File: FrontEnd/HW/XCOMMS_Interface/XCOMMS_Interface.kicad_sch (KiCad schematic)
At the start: 38 parts, among them J1 TFC-110-02-F-D-A-P-FR, J2 PicoBlade01x05, J3 PicoBlade01x05, J4 PicoBlade01x02, U1 STM32L431KBUx, U11 STM32L053R8Tx, Y1 ECS-.327-7-34QCS-TR

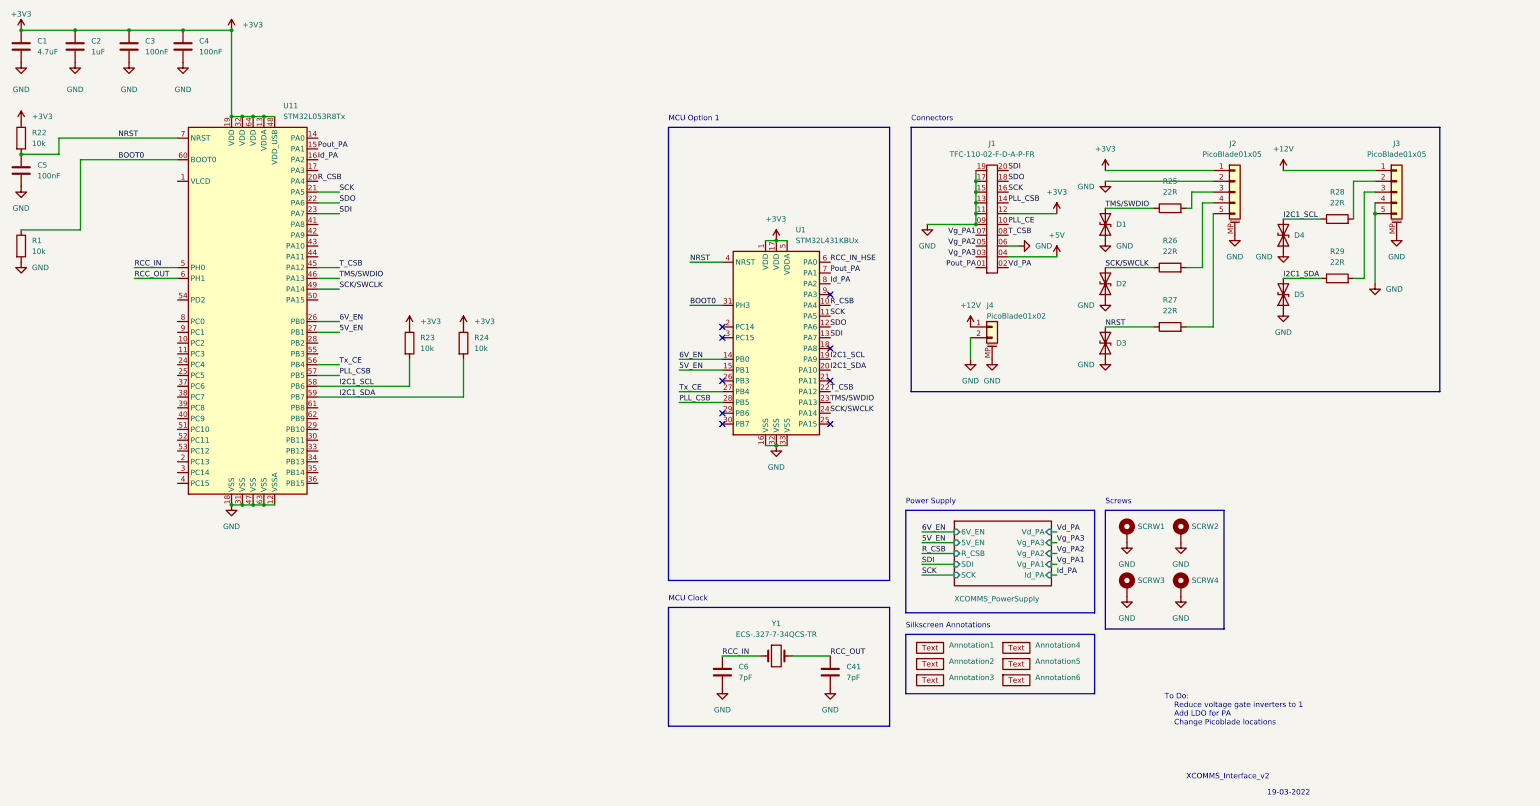
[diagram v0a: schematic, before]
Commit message: XCOMMS RF
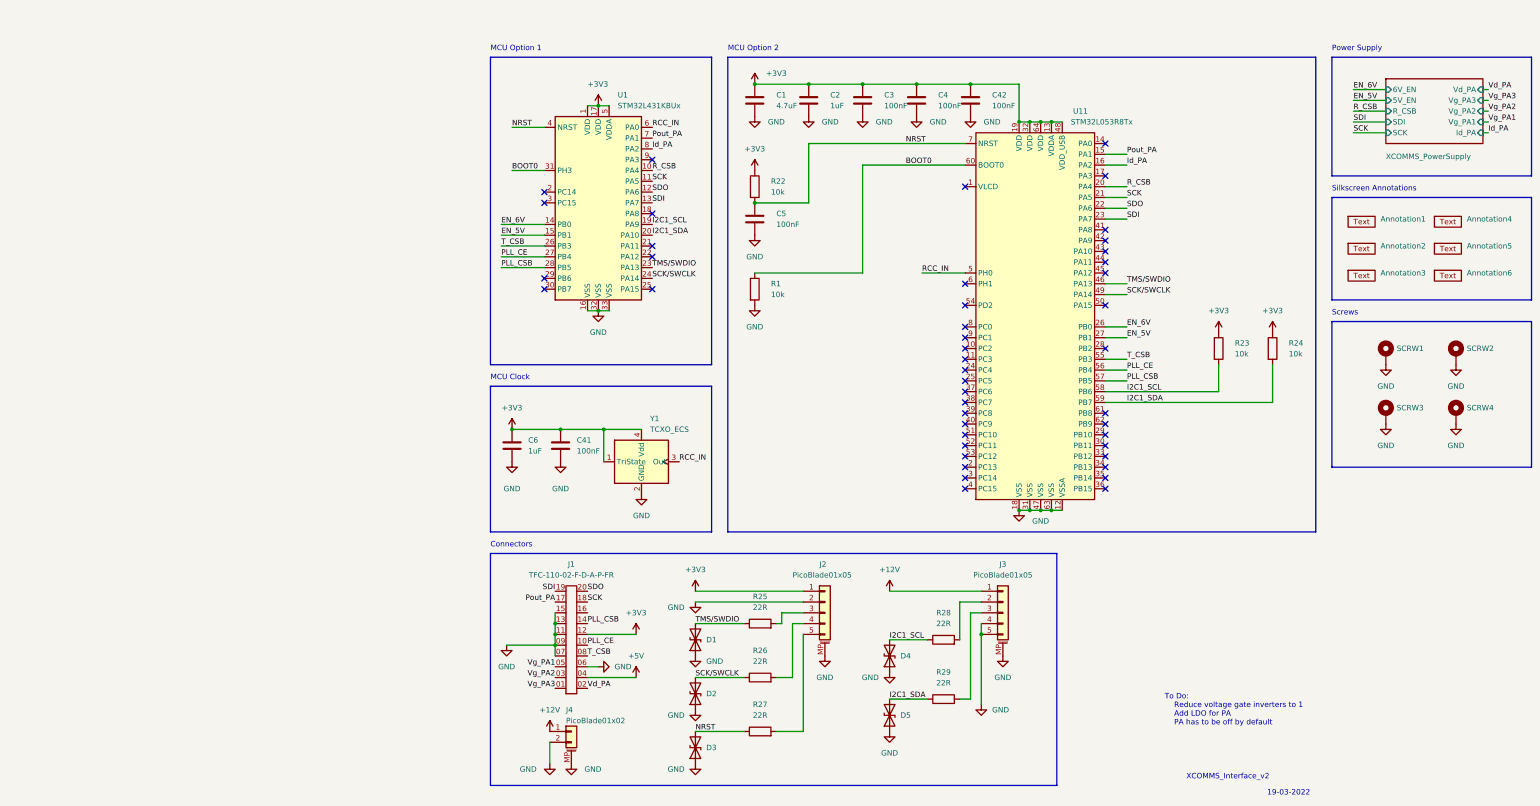
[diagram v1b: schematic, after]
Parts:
- removed Y1: ECS-.327-7-34QCS-TR, Crystal:Crystal_SMD_3215-2Pin_3.2x1.5mm, symbol Device:Crystal
- added C42: 100nF, Capacitor_SMD:C_0603_1608Metric, symbol Device:C
- added Y1: TCXO_ECS, GGS_Miscellaneous:TCXO_ECS, symbol GGS_Miscellaneous:TCXO_ECS
- C41: value 7pF -> 100nF
- C6: value 7pF -> 1uF
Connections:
- net RCC_IN_HSE is gone; now on net RCC_IN: U1.6 (PA0)
- net Tx_CE is gone; now on net PLL_CE: U1.27 (PB4), U11.56 (PB4)
- net +3V3: now also C41.1, C6.1, C42.1, Y1.1 (TriState), Y1.4 (Vdd)
- net GND: now also J1.07, C42.2, Y1.2 (GND); no longer J1.17, J1.19
- net Pout_PA: now also J1.17; no longer J1.01
- net RCC_IN: now also Y1.3 (Out); no longer C6.1
- net SCK: now also J1.18; no longer J1.16
- net SDI: now also J1.19; no longer J1.20
- net SDO: now also J1.20; no longer J1.18
- net T_CSB: now also U1.26 (PB3), U11.55 (PB3); no longer U1.22 (PA12), U11.45 (PA12)
- net Vg_PA1: now also J1.05; no longer J1.07
- net Vg_PA2: now also J1.03; no longer J1.05
- net Vg_PA3: now also J1.01; no longer J1.03
- net 5V_EN renamed EN_5V
- net 6V_EN renamed EN_6V
- net RCC_OUT: no longer names the net of U11.6 (PH1)
- net RCC_OUT: no longer C41.1
- no-connect marks 9 -> 45
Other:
- note added: "MCU Option 2"
- note added: "To Do: Reduce voltage gate inverters to 1 Add LDO for PA PA has to be off by default"
- note removed: "To Do: Reduce voltage gate inverters to 1 Add LDO for PA Change Picoblade locations"
- moved on the sheet: Annotation1, Annotation2, Annotation3, Annotation4, Annotation5, Annotation6, C1, C2, C3, C4, C5, D1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
